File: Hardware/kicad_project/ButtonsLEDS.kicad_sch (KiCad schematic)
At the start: 88 parts, among them SW10 spst_4_pin_internal, SW11 spst_4_pin_internal, SW12 spst_4_pin_internal, SW13 spst_4_pin_internal, SW14 spst_4_pin_internal, SW15 spst_4_pin_internal, SW16 spst_4_pin_internal, SW17 spst_4_pin_internal, SW18 spst_4_pin_internal, SW19 spst_4_pin_internal, SW2 spst_4_pin_internal, SW20 spst_4_pin_internal, SW21 spst_4_pin_internal, SW22 spst_4_pin_internal, SW23 spst_4_pin_internal, SW24 spst_4_pin_internal, SW25 spst_4_pin_internal, SW3 spst_4_pin_internal, SW4 spst_4_pin_internal, SW5 spst_4_pin_internal, SW6 spst_4_pin_internal, SW7 spst_4_pin_internal, SW8 spst_4_pin_internal, SW9 spst_4_pin_internal

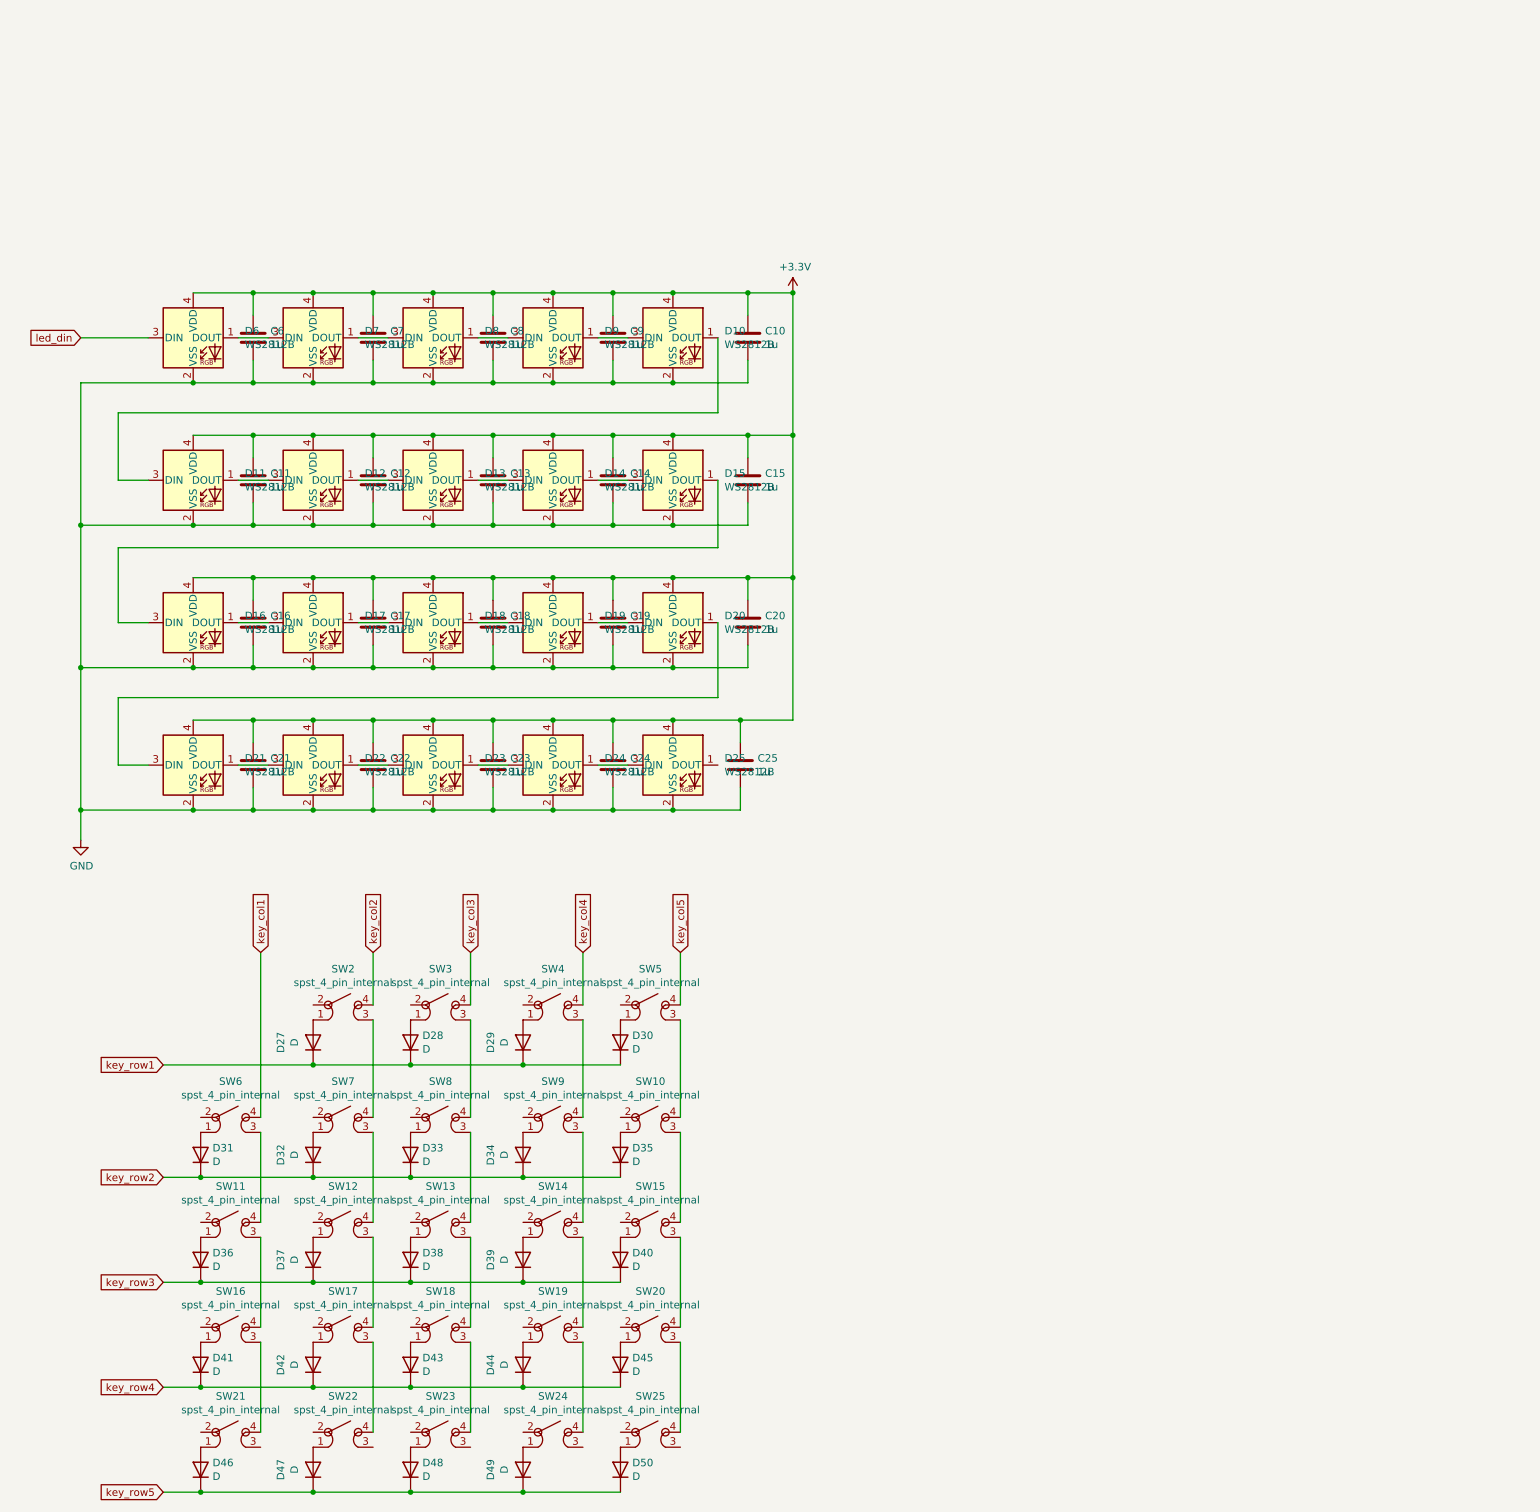
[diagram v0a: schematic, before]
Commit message: v9 hardware
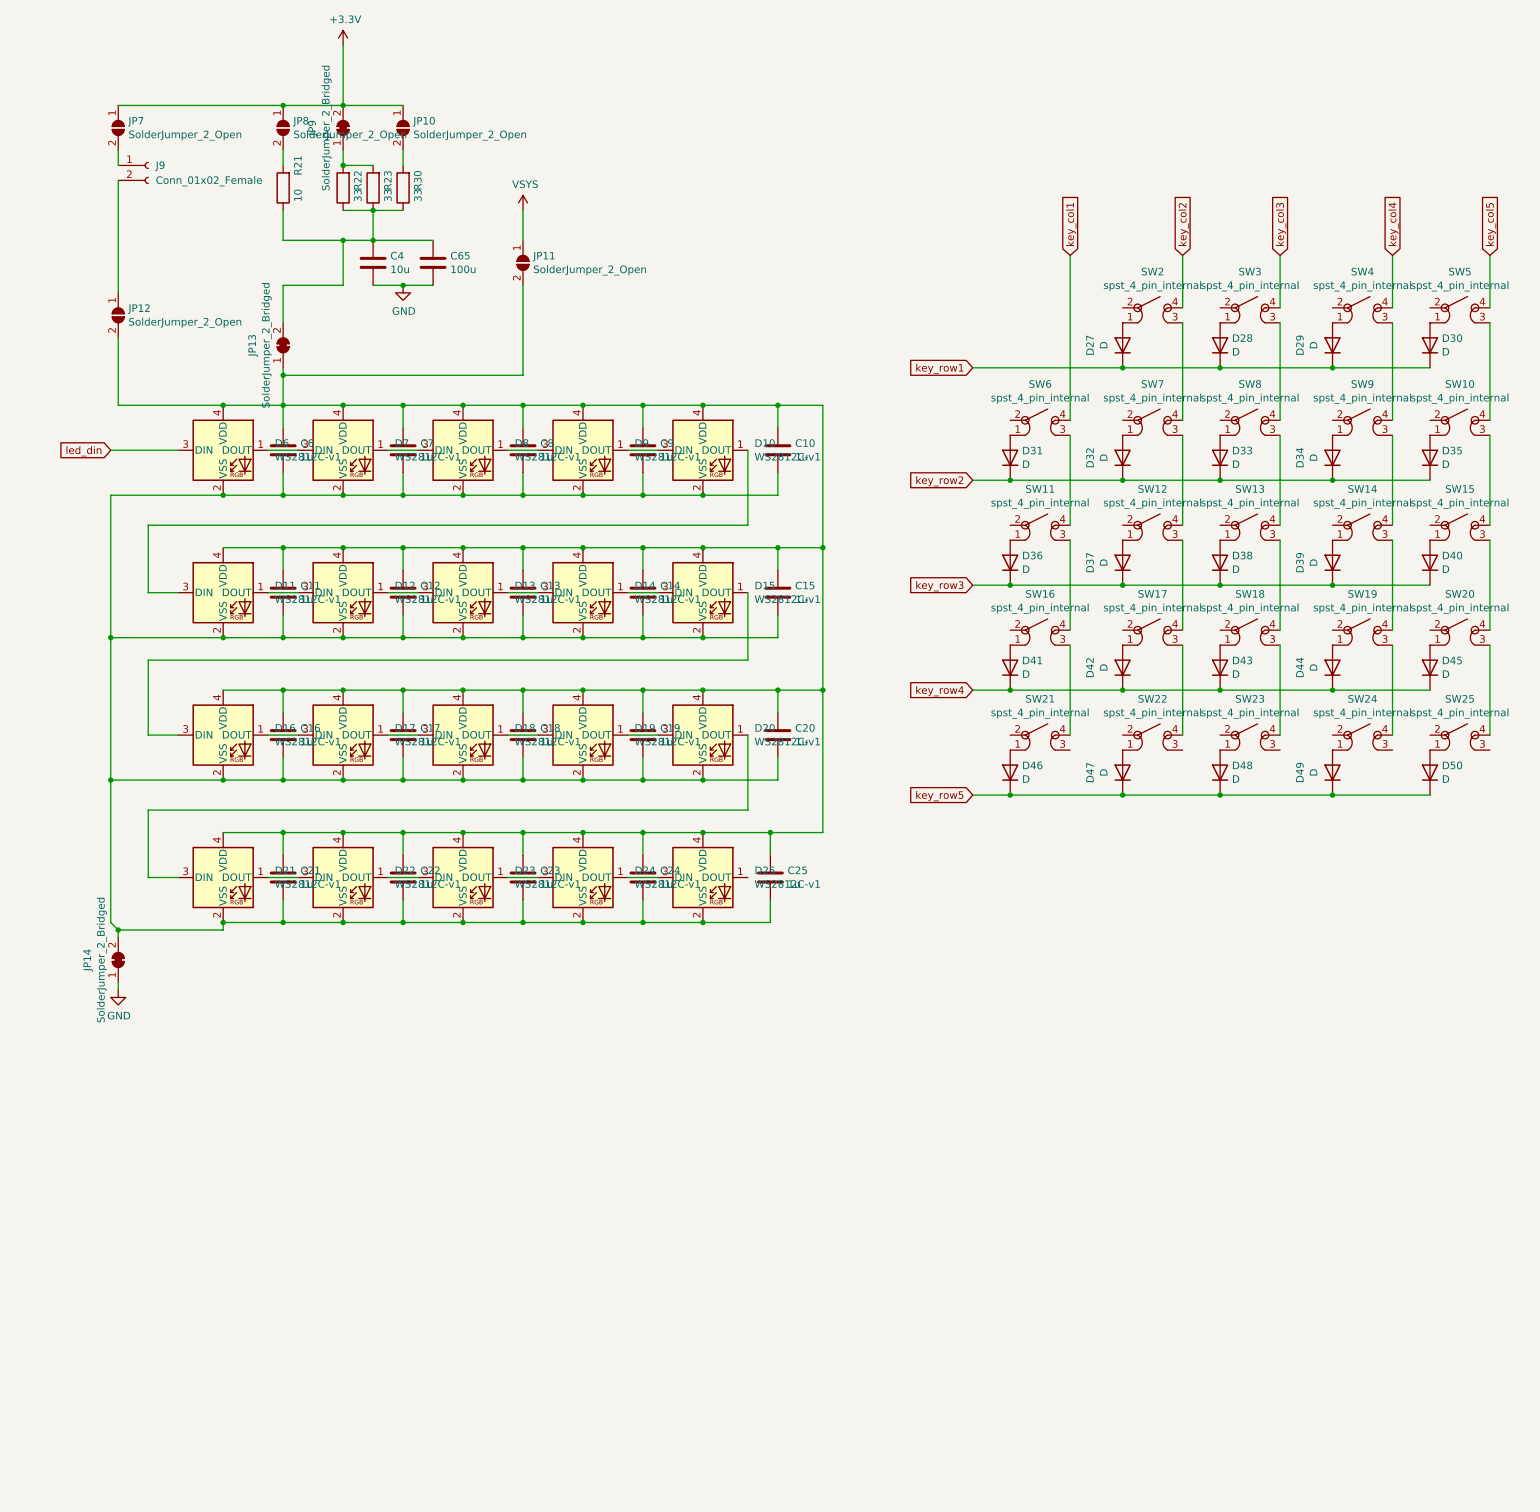
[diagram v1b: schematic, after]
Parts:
- added C4: 10u, Capacitors_SMD:C_0402_NoSilk, symbol Device:C
- added C65: 100u, Capacitor_Tantalum_SMD:CP_EIA-3528-21_Kemet-B, symbol Device:C
- added J9: Conn_01x02_Female, Connector_PinHeader_2.54mm:PinHeader_1x02_P2.54mm_Vertical, symbol Connector:Conn_01x02_Female
- added JP10, JP11, JP12, JP7, JP8: SolderJumper_2_Open, Jumper:SolderJumper-2_P1.3mm_Open_RoundedPad1.0x1.5mm, symbol Jumper:SolderJumper_2_Open
- added JP13, JP14, JP9: SolderJumper_2_Bridged, Jumper:SolderJumper-2_P1.3mm_Bridged_Pad1.0x1.5mm, symbol Jumper:SolderJumper_2_Bridged
- added R21: 10, Resistors_SMD:R_0402_NoSilk, symbol Device:R
- added R22, R23, R30: 33, Resistors_SMD:R_0402_NoSilk, symbol Device:R
- D10, D11, D12, D13, D14, D15, D16, D17, D18, D19, D20, D21, D22, D23, D24, D25, D6, D7, D8, D9: value WS2812B -> WS2812C-v1; LCSC C965556 -> C2976072
- D27, D28, D29, D30, D31, D32, D33, D34, D35, D36, D37, D38, D39, D40, D41, D42, D43, D44, D45, D46, D47, D48, D49, D50: LCSC c2128 -> C2128
- SW10, SW11, SW12, SW13, SW14, SW15, SW16, SW17, SW18, SW19, SW2, SW20, SW21, SW22, SW23, SW24, SW25, SW3, SW4, SW5, SW6, SW7, SW8, SW9: footprint RandomJunk:ts1102_smallerpads_buttonhole -> MyLibrary:ts1187; LCSC C480275 -> C318884
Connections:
- net +3V3: now also JP10.1 (A), JP7.1 (A), JP8.1 (A), JP9.2 (B); no longer C10.1, C11.1, C12.1, C13.1, C14.1, C15.1, C16.1, C17.1, C18.1, C19.1, C20.1, C21.1, C22.1, C23.1, C24.1, C25.1, C6.1, C7.1, C8.1, C9.1, D10.4 (VDD), D11.4 (VDD), D12.4 (VDD), D13.4 (VDD), D14.4 (VDD), D15.4 (VDD), D16.4 (VDD), D17.4 (VDD), D18.4 (VDD), D19.4 (VDD), D20.4 (VDD), D21.4 (VDD), D22.4 (VDD), D23.4 (VDD), D24.4 (VDD), D25.4 (VDD), D6.4 (VDD), D7.4 (VDD), D8.4 (VDD), D9.4 (VDD)
- net GND: now also C4.2, C65.2, JP14.1 (A); no longer C10.2, C11.2, C12.2, C13.2, C14.2, C15.2, C16.2, C17.2, C18.2, C19.2, C20.2, C21.2, C22.2, C23.2, C24.2, C25.2, C6.2, C7.2, C8.2, C9.2, D10.2 (VSS), D11.2 (VSS), D12.2 (VSS), D13.2 (VSS), D14.2 (VSS), D15.2 (VSS), D16.2 (VSS), D17.2 (VSS), D18.2 (VSS), D19.2 (VSS), D20.2 (VSS), D21.2 (VSS), D22.2 (VSS), D23.2 (VSS), D24.2 (VSS), D25.2 (VSS), D6.2 (VSS), D7.2 (VSS), D8.2 (VSS), D9.2 (VSS)
- new net: C10.1, C11.1, C12.1, C13.1, C14.1, C15.1, C16.1, C17.1, C18.1, C19.1, C20.1, C21.1, C22.1, C23.1, C24.1, C25.1, C6.1, C7.1, C8.1, C9.1, D10.4 (VDD), D11.4 (VDD), D12.4 (VDD), D13.4 (VDD), D14.4 (VDD), D15.4 (VDD), D16.4 (VDD), D17.4 (VDD), D18.4 (VDD), D19.4 (VDD), D20.4 (VDD), D21.4 (VDD), D22.4 (VDD), D23.4 (VDD), D24.4 (VDD), D25.4 (VDD), D6.4 (VDD), D7.4 (VDD), D8.4 (VDD), D9.4 (VDD), JP11.2 (B), JP12.2 (B), JP13.1 (A)
- new net: C10.2, C11.2, C12.2, C13.2, C14.2, C15.2, C16.2, C17.2, C18.2, C19.2, C20.2, C21.2, C22.2, C23.2, C24.2, C25.2, C6.2, C7.2, C8.2, C9.2, D10.2 (VSS), D11.2 (VSS), D12.2 (VSS), D13.2 (VSS), D14.2 (VSS), D15.2 (VSS), D16.2 (VSS), D17.2 (VSS), D18.2 (VSS), D19.2 (VSS), D20.2 (VSS), D21.2 (VSS), D22.2 (VSS), D23.2 (VSS), D24.2 (VSS), D25.2 (VSS), D6.2 (VSS), D7.2 (VSS), D8.2 (VSS), D9.2 (VSS), JP14.2 (B)
- new net: C4.1, C65.1, JP13.2 (B), R21.1, R22.1, R23.1, R30.1
- new net: JP10.2 (B), R30.2
- new net: J9.2 (Pin_2), JP12.1 (A)
- new net: JP9.1 (A), R22.2, R23.2
- new net: J9.1 (Pin_1), JP7.2 (B)
- new net: JP8.2 (B), R21.2
- new net VBUS: JP11.1 (A)
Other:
- moved on the sheet: C10, C11, C12, C13, C14, C15, C16, C17, C18, C19, C20, C21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

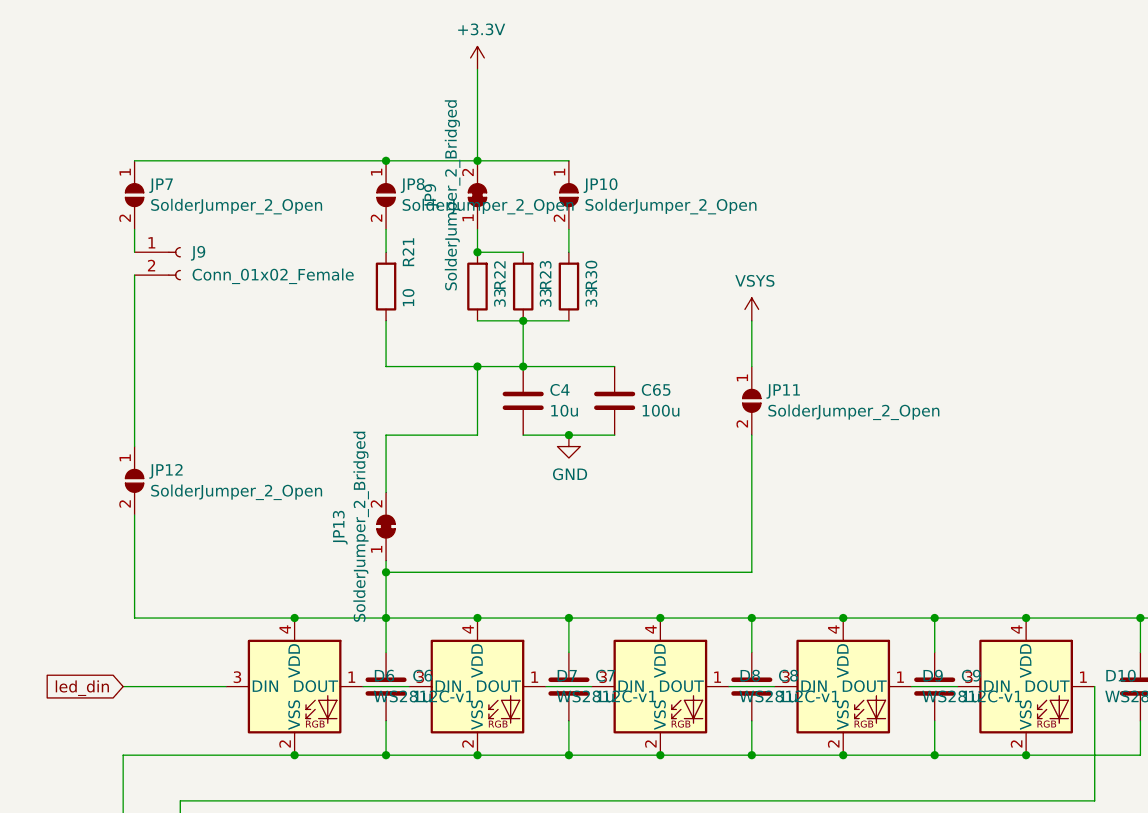
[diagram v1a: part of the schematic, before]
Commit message: v10 board
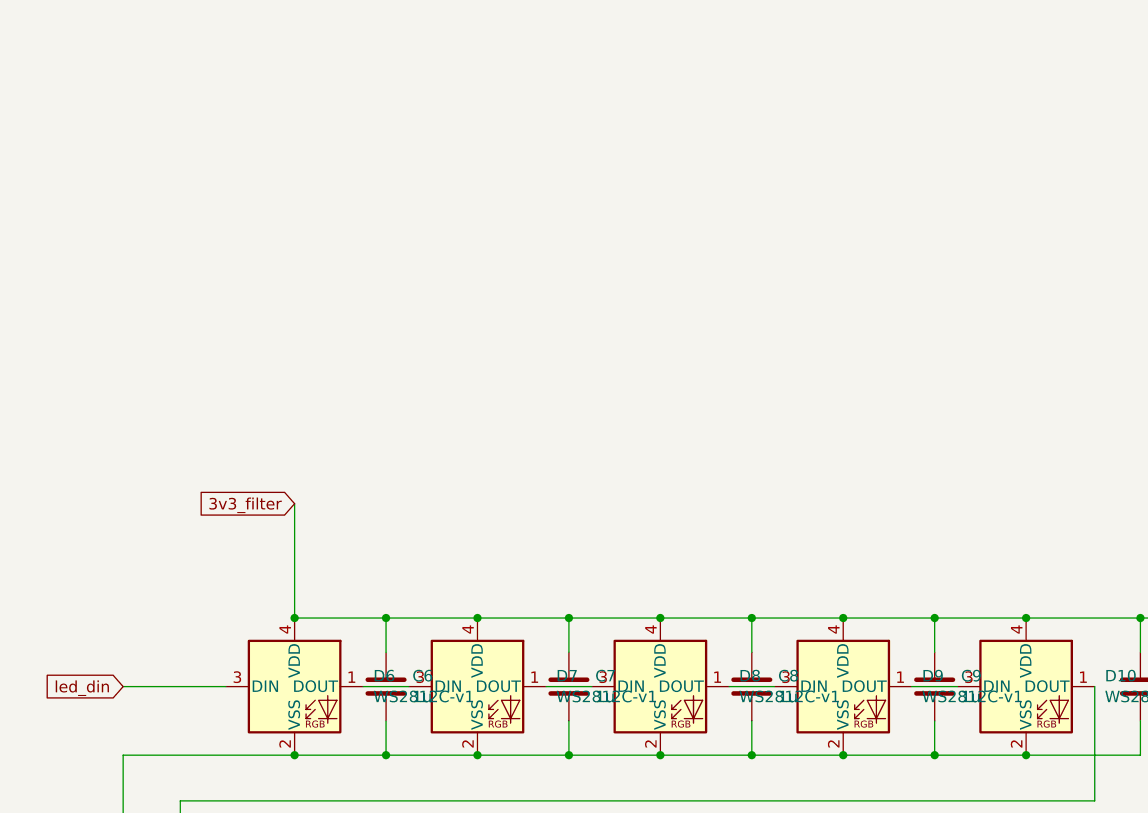
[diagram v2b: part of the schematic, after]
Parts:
- removed C4: 10u, Capacitors_SMD:C_0402_NoSilk, symbol Device:C
- removed C65: 100u, Capacitor_Tantalum_SMD:CP_EIA-3528-21_Kemet-B, symbol Device:C
- removed J9: Conn_01x02_Female, Connector_PinHeader_2.54mm:PinHeader_1x02_P2.54mm_Vertical, symbol Connector:Conn_01x02_Female
- removed JP10, JP11, JP12, JP7, JP8: SolderJumper_2_Open, Jumper:SolderJumper-2_P1.3mm_Open_RoundedPad1.0x1.5mm, symbol Jumper:SolderJumper_2_Open
- removed JP13, JP9: SolderJumper_2_Bridged, Jumper:SolderJumper-2_P1.3mm_Bridged_Pad1.0x1.5mm, symbol Jumper:SolderJumper_2_Bridged
- removed R21: 10, Resistors_SMD:R_0402_NoSilk, symbol Device:R
- removed R22, R23, R30: 33, Resistors_SMD:R_0402_NoSilk, symbol Device:R
- C10, C11, C12, C13, C14, C15, C16, C17, C18, C19, C20, C21, C22, C23, C24, C25, C6, C7, C8, C9: footprint Capacitors_SMD:C_0402_NoSilk -> Capacitor_SMD:C_0402_1005Metric; checked (none) -> 1
- D10, D11, D12, D13, D14, D15, D16, D17, D18, D19, D20, D21, D22, D23, D24, D25, D27, D28, D29, D30, D31, D32, D33, D34, D35, D36, D37, D38, D39, D40, D41, D42, D43, D44, D45, D46, D47, D48, D49, D50, D6, D7, D8, D9, SW10, SW11, SW12, SW13, SW14, SW15, SW16, SW17, SW18, SW19, SW2, SW20, SW21, SW22, SW23, SW24, SW25, SW3, SW4, SW5, SW6, SW7, SW8, SW9: checked (none) -> 1
- JP14: checked 1 -> (none)
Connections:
- net 3v3_filter: now reaches C10.1, C11.1, C12.1, C13.1, C14.1, C15.1, C16.1, C17.1, C18.1, C19.1, C20.1, C21.1, C22.1, C23.1, C24.1, C25.1, C6.1, C7.1, C8.1, C9.1, D10.4 (VDD), D11.4 (VDD), D12.4 (VDD), D13.4 (VDD), D14.4 (VDD), D15.4 (VDD), D16.4 (VDD), D17.4 (VDD), D18.4 (VDD), D19.4 (VDD), D20.4 (VDD), D21.4 (VDD), D22.4 (VDD), D23.4 (VDD), D24.4 (VDD), D25.4 (VDD), D6.4 (VDD), D7.4 (VDD), D8.4 (VDD), D9.4 (VDD)
